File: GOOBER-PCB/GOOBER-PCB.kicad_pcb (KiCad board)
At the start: 2 copper layers, 78 x 101 mm, 88 parts, among them J1 XT30U_F, J2 Conn_01x22, J3 Conn_01x22, J4 Conn_01x22, J5 Conn_01x22, J6 XT30U_F, J8 USB C vertical, Q3 PJD15P06A_L2_00001, Q4 AO3419, U1 TPS565208

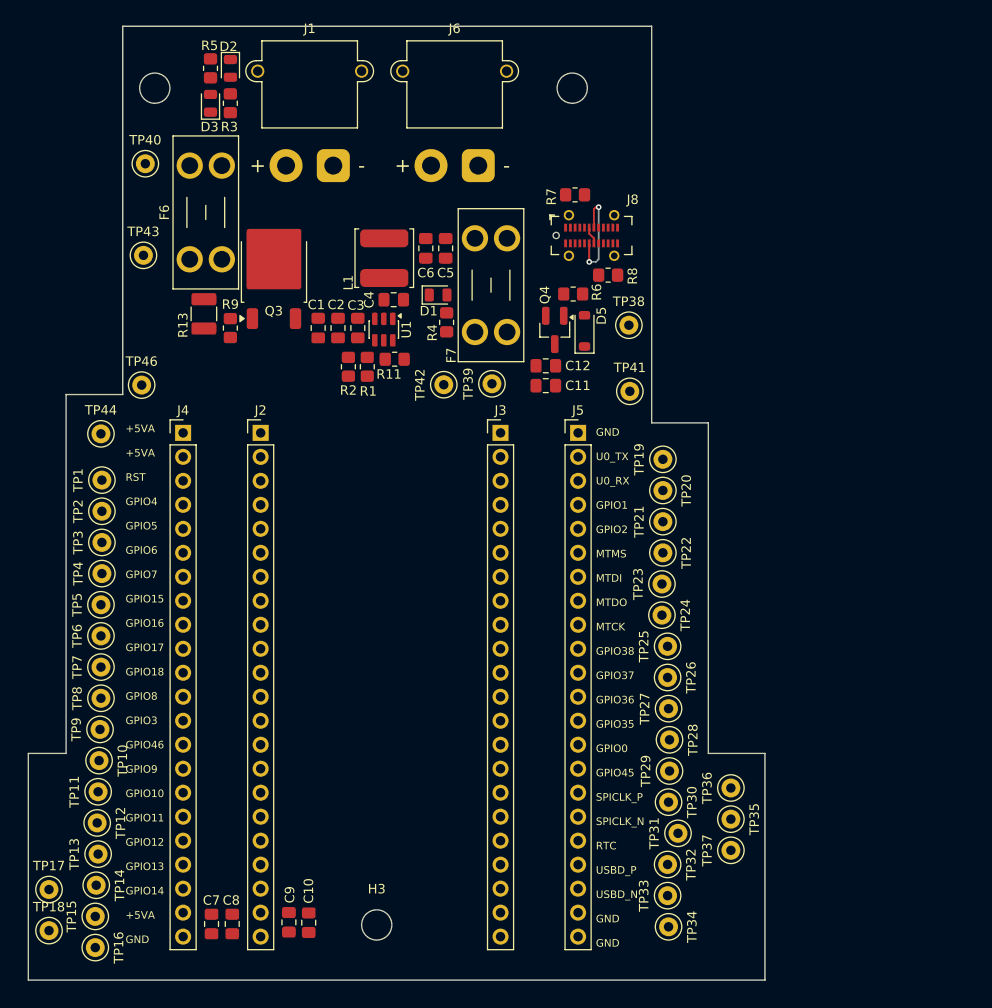
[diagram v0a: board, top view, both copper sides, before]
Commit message: some work on pcb
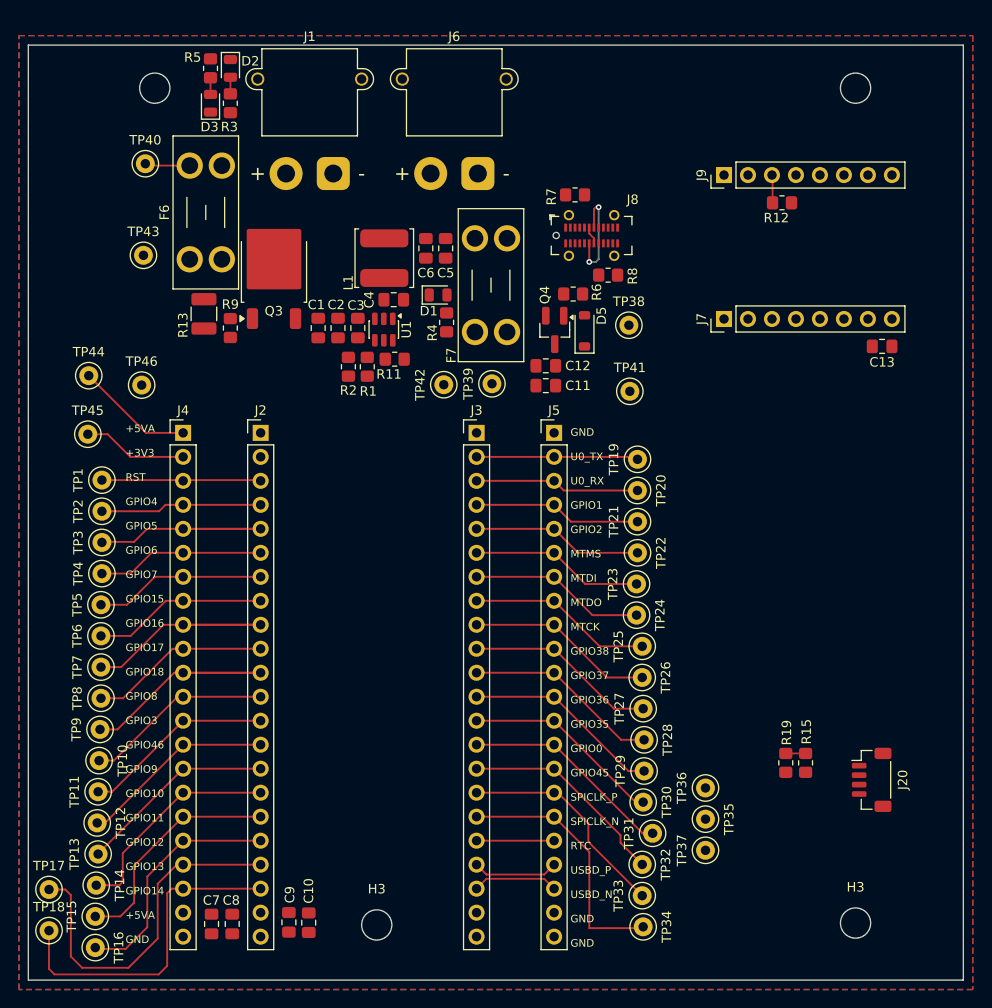
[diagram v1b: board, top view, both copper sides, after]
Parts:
- added C13: 0.1uF, Capacitor_SMD:C_0805_2012Metric_Pad1.18x1.45mm_HandSolder, F.Cu at (111.4, 48.9)
- added H3: MountingHole, MountingHole:MountingHole_3.2mm_M3_ISO7380, F.Cu at (108.6, 110.0)
- added J20: BM04B-SRSS-TB, Connector_JST:JST_SH_BM04B-SRSS-TB_1x04-1MP_P1.00mm_Vertical, F.Cu at (110.3, 94.8)
- added J7: Conn_01x08, Connector_PinHeader_2.54mm:PinHeader_1x08_P2.54mm_Vertical, F.Cu at (94.7, 46.0)
- added J9: Conn_01x08, Connector_PinHeader_2.54mm:PinHeader_1x08_P2.54mm_Vertical, F.Cu at (94.7, 30.8)
- added R12: 10K, Resistor_SMD:R_0805_2012Metric_Pad1.20x1.40mm_HandSolder, F.Cu at (100.8, 33.7)
- added R15: 10K, Resistor_SMD:R_0805_2012Metric_Pad1.20x1.40mm_HandSolder, F.Cu at (103.3, 93.0)
- added R19: 10K, Resistor_SMD:R_0805_2012Metric_Pad1.20x1.40mm_HandSolder, F.Cu at (101.2, 93.0)
- added TP45: TP, TestPoint:TestPoint_Keystone_5000-5004_Miniature, F.Cu at (27.3, 58.2)
- moved H2 30.0 mm to (108.6, 21.6)
- moved TP44 6.29 mm to (27.4, 52.0)
- moved TP27 2.69 mm to (86.1, 87.3)
- moved TP30 2.69 mm to (86.1, 97.2)
- moved TP31 2.69 mm to (87.1, 100.5)
- moved TP34 2.69 mm to (86.1, 110.4)
- moved TP19 2.69 mm to (85.5, 60.9)
- moved TP20 2.69 mm to (85.5, 64.2)
- moved TP21 2.69 mm to (85.5, 67.5)
- moved TP22 2.69 mm to (85.5, 70.8)
- moved TP23 2.69 mm to (85.4, 74.1)
- moved TP24 2.69 mm to (85.4, 77.4)
- moved TP25 2.69 mm to (86.0, 80.7)
- moved TP26 2.69 mm to (86.0, 84.0)
- moved TP28 2.69 mm to (86.2, 90.6)
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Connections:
- net MTCK renamed CLK
- net MTDI renamed MOSI
- net MTDO renamed MISO
- net MTMS renamed CS
- J2 pad 1: unconnected-(J2-Pin_1-Pad1) -> +3V3
- J2 pad 2: unconnected-(J2-Pin_2-Pad2) -> +3V3
- J4 pad 2: +5VA -> +3V3
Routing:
- net GPIO13: track 0.00 -> 37.6 mm
- net GPIO14: track 0.00 -> 35.0 mm
- net GPIO18: track 0.00 -> 27.7 mm
- net SPICLK_N: track 0.00 -> 27.3 mm
- net GPIO16: track 0.00 -> 27.0 mm
- net GPIO5: track 0.00 -> 25.6 mm
- net GPIO12: track 0.00 -> 25.5 mm
- net GPIO11: track 0.00 -> 24.2 mm
- net GPIO10: track 0.00 -> 23.3 mm
- net SPICLK_P: track 0.00 -> 23.2 mm
- net GPIO0: track 0.00 -> 22.5 mm
- net GPIO45: track 0.00 -> 22.2 mm
- net CS: track 0.00 -> 21.3 mm
- net GPIO35: track 0.00 -> 21.2 mm
- net GPIO36: track 0.00 -> 21.0 mm
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- added copper zone on B.Cu, net GND
- added copper zone on F.Cu, net GND
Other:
- board size 78 x 101 mm -> 99 x 99 mm
- board text added: "+5VA +3V3 RST GPIO4 GPIO5 GPIO6 GPIO7 GPIO15 GPIO16 GPIO17 GPIO18 GPIO8 GPIO3 GPIO46 GPIO9 GPIO10 GPIO11 GPIO12 GPIO13 GPIO14 +5VA GND"
- board text removed: "+5VA +5VA RST GPIO4 GPIO5 GPIO6 GPIO7 GPIO15 GPIO16 GPIO17 GPIO18 GPIO8 GPIO3 GPIO46 GPIO9 GPIO10 GPIO11 GPIO12 GPIO13 GPIO14 +5VA GND"
